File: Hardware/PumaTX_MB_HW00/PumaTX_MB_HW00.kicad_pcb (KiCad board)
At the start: 2 copper layers, 216 x 107.5 mm, 107 parts, among them J100 FH12A-26S-0.5SH_55_, J101 FH12-12S-0.5SH_55_, J102 500334-0160, J103 500334-0160, J104 692122030100, J105 53398-0667, J300 U.FL-R-SMT-1_40_, J410 U.FL-R-SMT-1_40_, M130 Motor_DC, M140 Fan, Q130 ZXMN3B01F, Q140 ZXMN3B01F, Q200 UMH3NTN, Q201 UMH3NTN, U200 CP2105-F01-GMR, U300 ESP32-PICO-D4, U400 ESP32-PICO-D4, U402 E28-2G4M27S, U410 SX1280, U500 BQ24075RGTR, U510 MIC5528-3.3YMT-T5, U520 MIC5528-3.3YMT-T5, U530 MIC5528-3.3YMT-T5, Y410 NX2016SA-52MHZ-EXS00A-CS06016

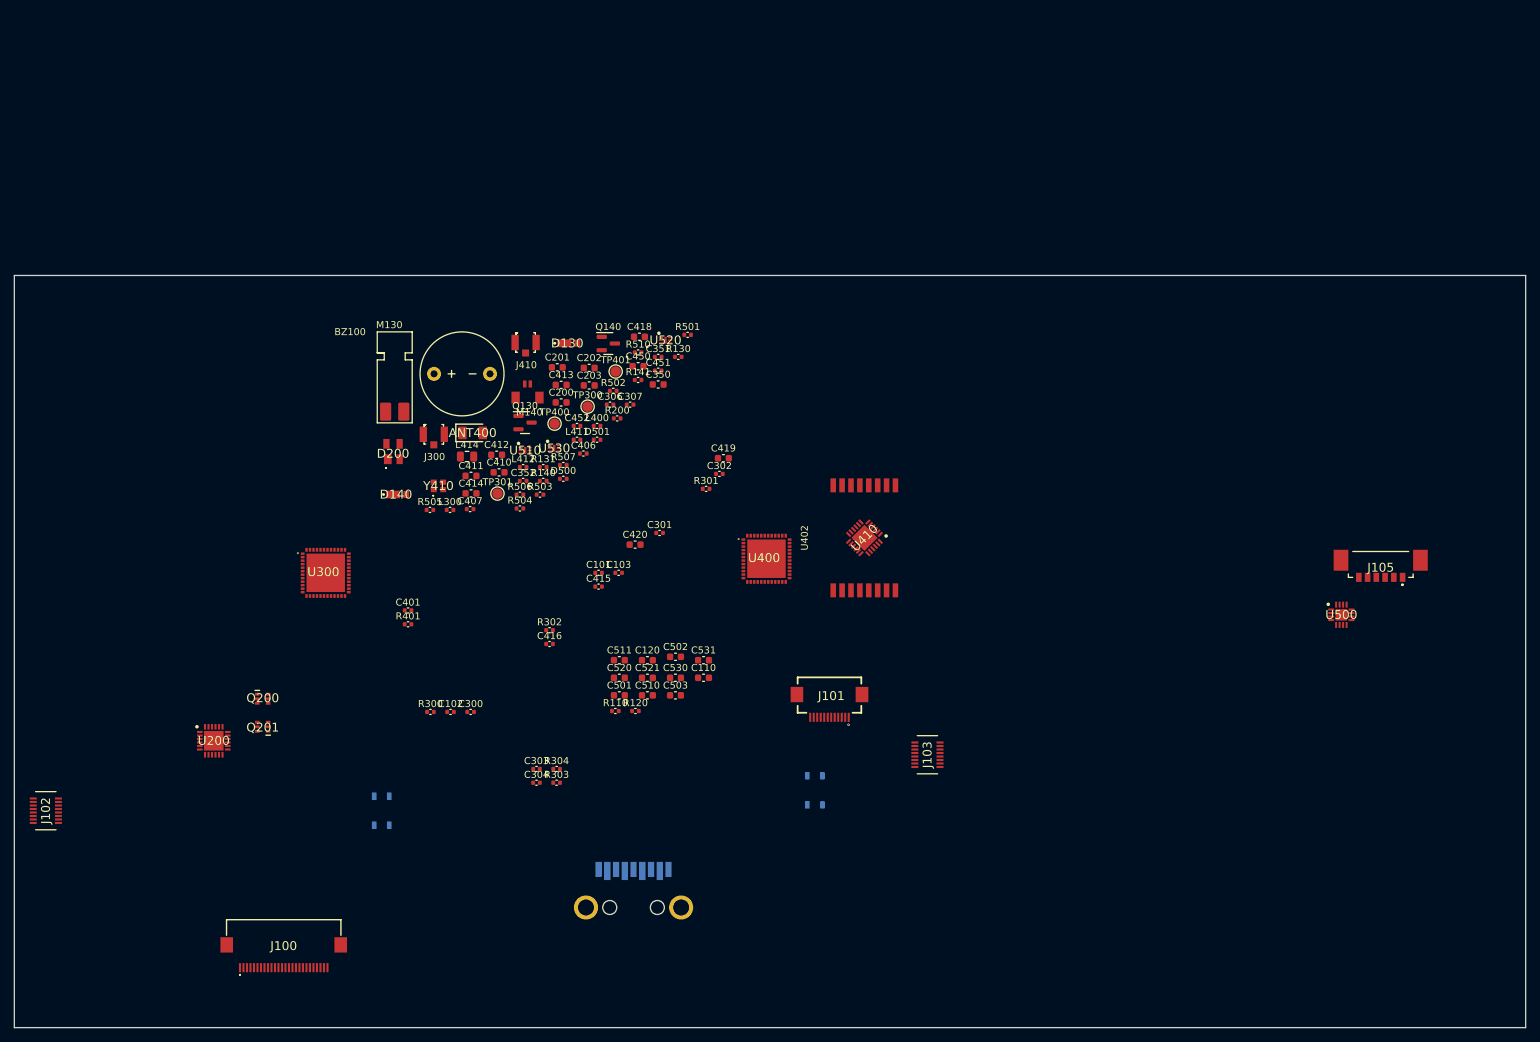
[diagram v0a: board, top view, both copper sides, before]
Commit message: PCB layout is done, routing to go!
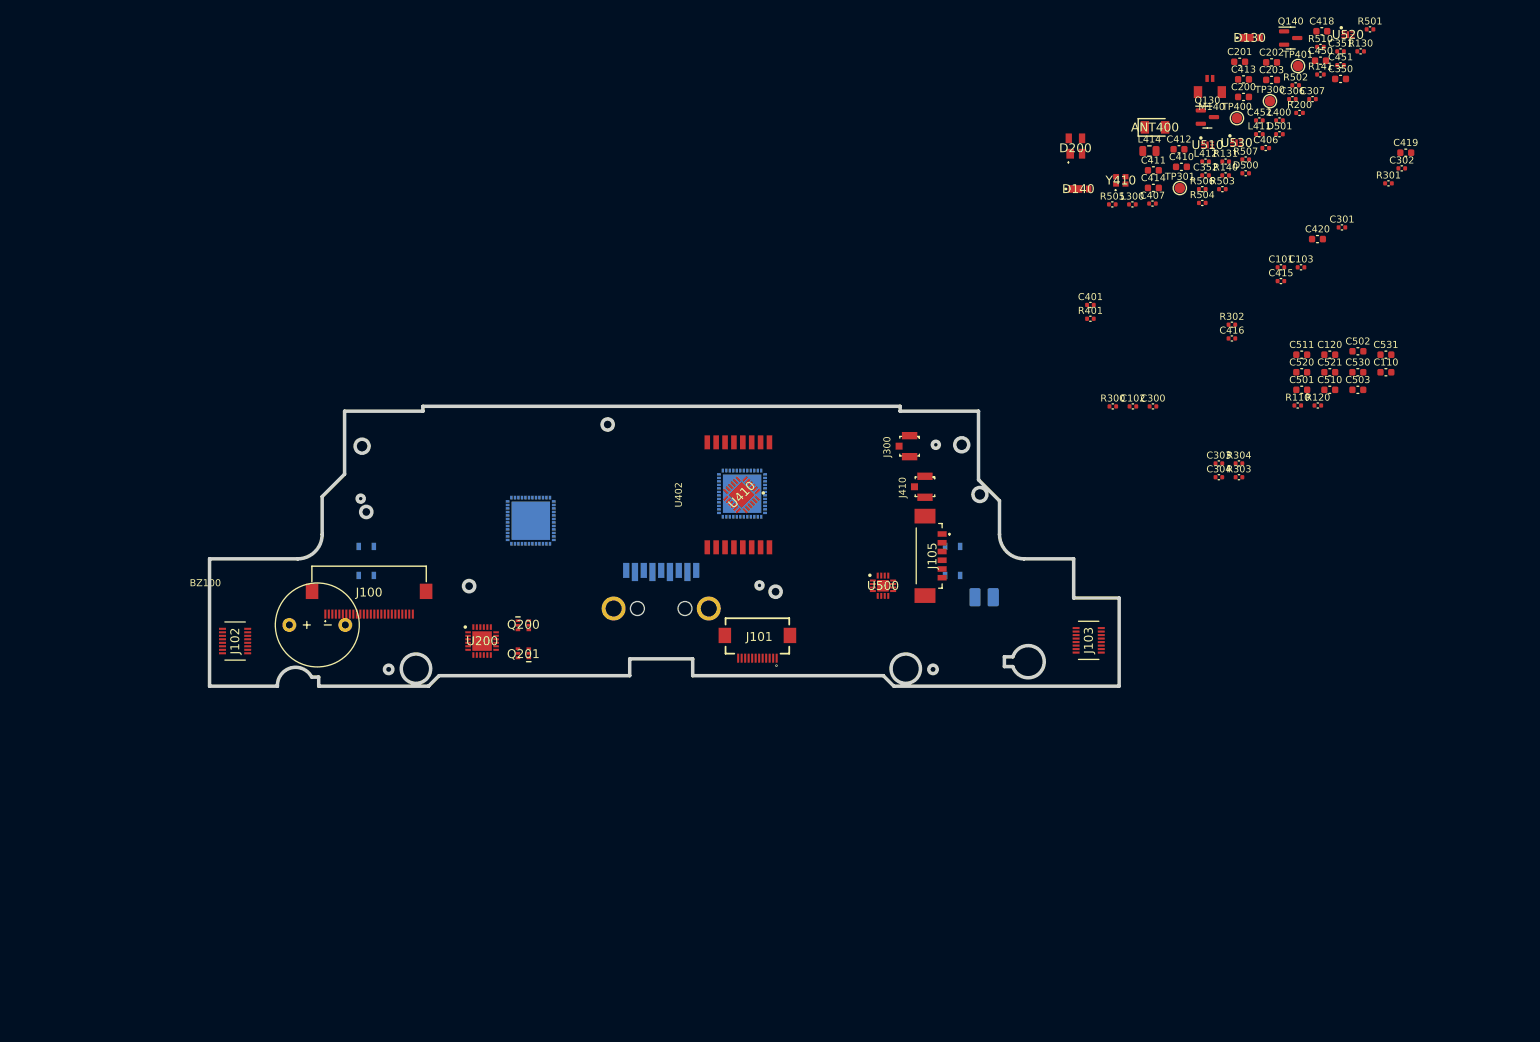
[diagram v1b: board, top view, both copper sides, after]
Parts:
- M130, U300, U400: moved to B.Cu
- moved ANT400 106.9 mm to (216.5, 43.3)
- moved C101 106.9 mm to (234.5, 63.3)
- moved C102 106.9 mm to (213.4, 83.2)
- moved C103 106.9 mm to (237.4, 63.3)
- moved C110 106.9 mm to (249.5, 78.3)
- moved C120 106.9 mm to (241.5, 75.8)
- moved C200 106.9 mm to (229.2, 39.0)
- moved C201 106.9 mm to (228.6, 34.0)
- moved C202 106.9 mm to (233.2, 34.0)
- moved C203 106.9 mm to (233.2, 36.6)
- moved C301 106.9 mm to (243.2, 57.6)
- moved C303 106.9 mm to (225.7, 91.4)
- moved C304 106.9 mm to (225.7, 93.3)
- moved C306 106.9 mm to (236.2, 39.3)
- moved C307 106.9 mm to (239.0, 39.3)
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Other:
- board size 216 x 107.5 mm -> 130 x 40 mm
